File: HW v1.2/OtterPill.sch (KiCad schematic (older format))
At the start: 39 parts, among them J1 USB-c, J2 VBUS, J3 1, J4 2, J5 SWD, J6 GND, J7 PAD, SW1 SW_Push, U1 USBLC6-4, U2 STM32F072C8Tx, U3 SY8201, U4 FUSB302BMPX

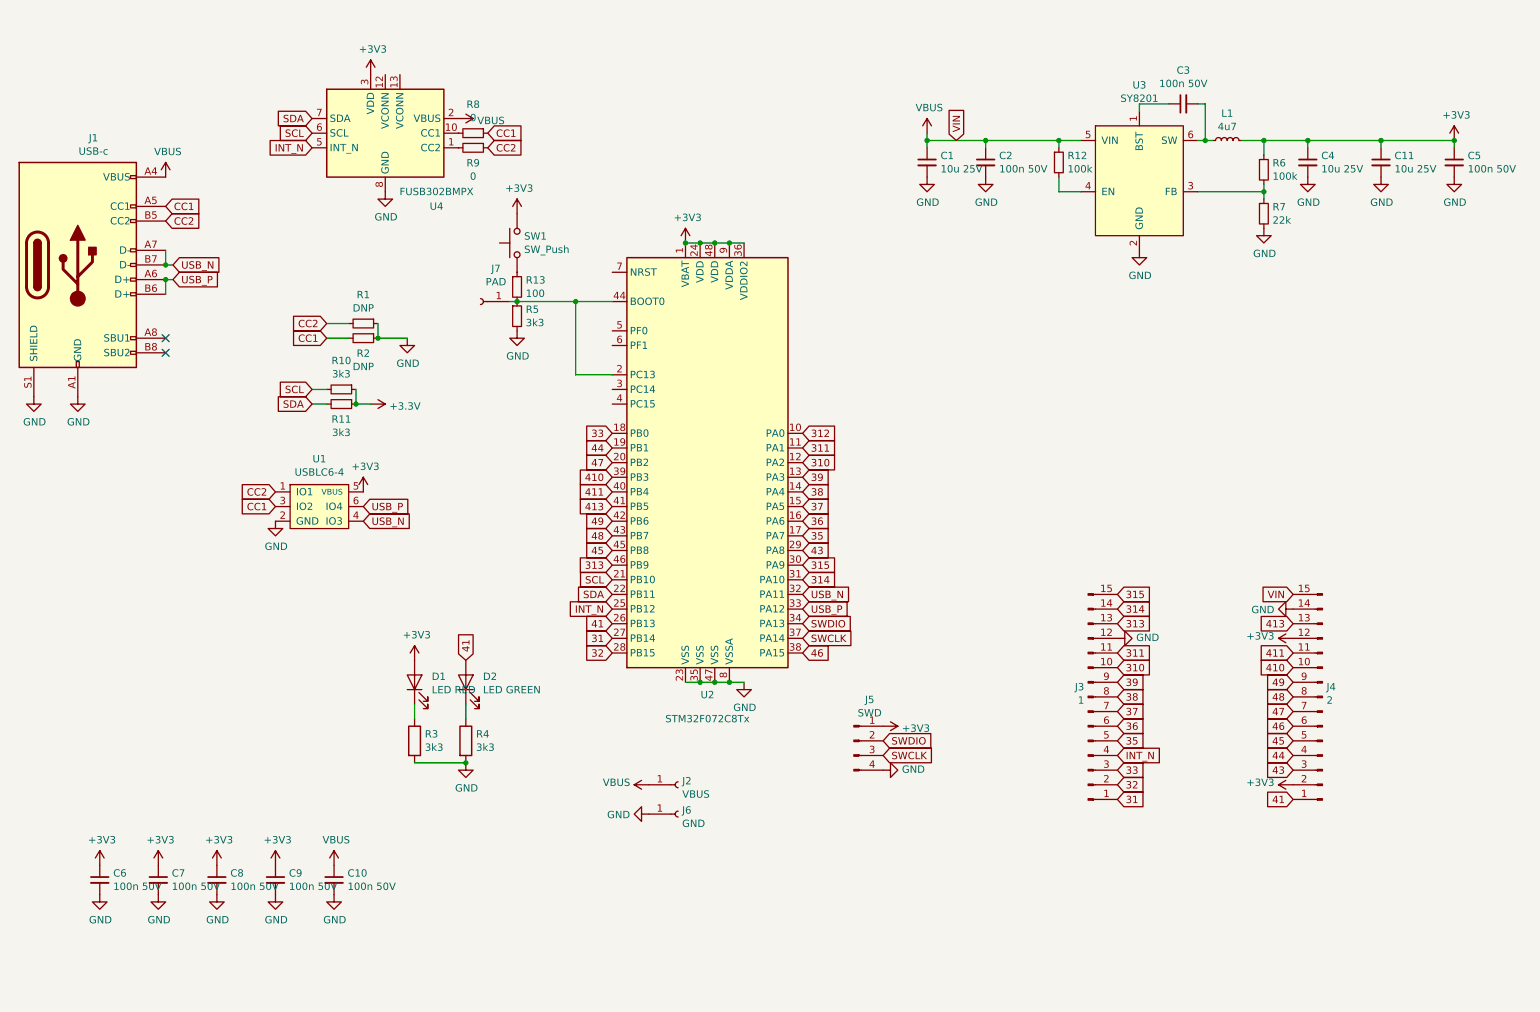
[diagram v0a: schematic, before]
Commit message: schematic cleanup
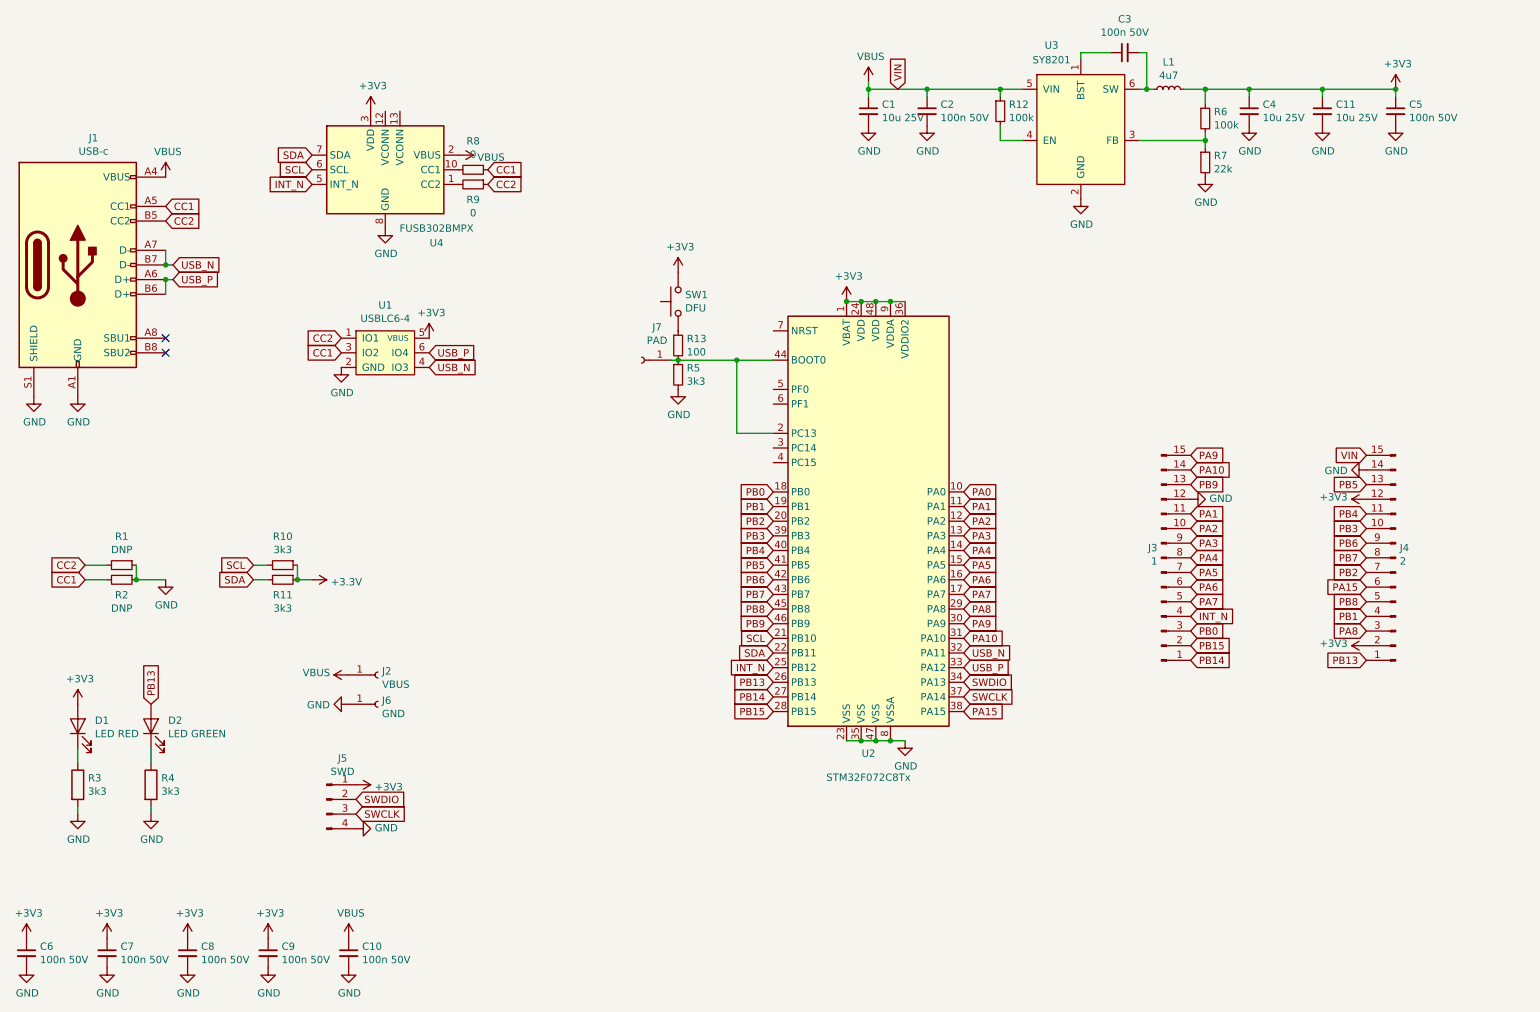
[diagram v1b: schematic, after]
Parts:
- SW1: value SW_Push -> DFU
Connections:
- net 31 renamed PB14
- net 310 renamed PA2
- net 311 renamed PA1
- net 312 renamed PA0
- net 313 renamed PB9
- net 314 renamed PA10
- net 315 renamed PA9
- net 32 renamed PB15
- net 33 renamed PB0
- net 35 renamed PA7
- net 36 renamed PA6
- net 37 renamed PA5
- net 38 renamed PA4
- net 39 renamed PA3
- net 41 renamed PB13
- net 410 renamed PB3
- net 411 renamed PB4
- net 413 renamed PB5
- net 43 renamed PA8
- net 44 renamed PB1
- net 45 renamed PB8
- net 46 renamed PA15
- net 47 renamed PB2
- net 48 renamed PB7
- net 49 renamed PB6
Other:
- moved on the sheet: C1, C10, C11, C2, C3, C4, C5, C6, C7, C8, C9, D1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
